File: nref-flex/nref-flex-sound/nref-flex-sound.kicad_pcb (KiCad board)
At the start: 2 copper layers, 6.5 x 115 mm, 3 parts, among them J1 Conn_01x10_Pin, J2 Conn_01x10_Pin

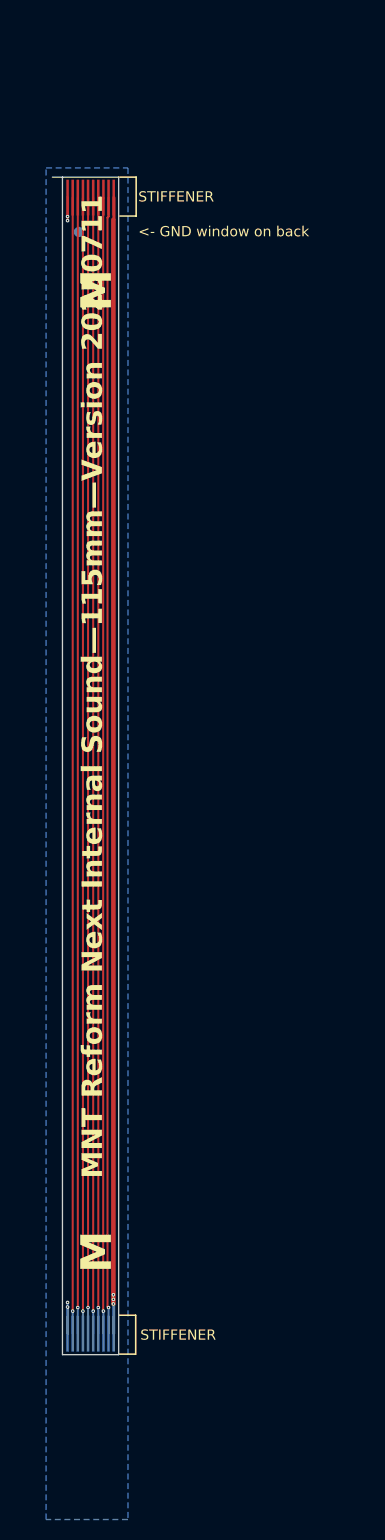
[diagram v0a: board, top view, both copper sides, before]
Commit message: commit various flex changes
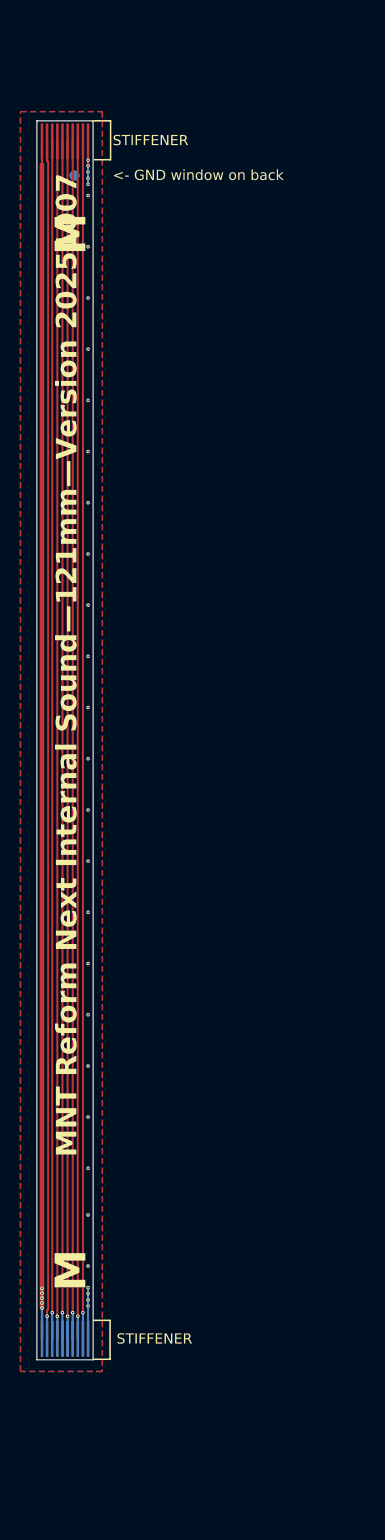
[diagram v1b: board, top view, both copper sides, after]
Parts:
- moved J1 6.04 mm to (85.7, 44.2), turned to 180 degrees
- moved TP1 5.53 mm to (86.6, 47.5)
- moved J2 2.55 mm to (85.7, 161.2), turned to 180 degrees
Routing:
- net +3V3: track 111.9 -> 118.7 mm, vias 3 -> 5
- net Net-(J1-Pin_8): track 111.0 -> 117.0 mm
- net Net-(J1-Pin_2): track 111.0 -> 117.0 mm
- net Net-(J1-Pin_9): track 111.0 -> 117.0 mm
- net Net-(J1-Pin_7): track 111.0 -> 117.0 mm
- net Net-(J1-Pin_6): track 111.0 -> 117.0 mm
- net Net-(J1-Pin_5): track 111.0 -> 117.0 mm
- net Net-(J1-Pin_4): track 111.0 -> 117.0 mm
- net Net-(J1-Pin_3): track 111.0 -> 117.0 mm
- net GND: track 8.10 -> 7.75 mm, vias 4 -> 31
- added copper zone on F.Cu, net GND
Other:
- board size 6.5 x 115 mm -> 5.5 x 121 mm
- board text added: "MNT Reform Next Internal Sound—121mm—Version 20251007"
- board text added: "target length: 121mm"
- board text removed: "MNT Reform Next Internal Sound—115mm—Version 20250711"
- board text removed: "trace w: 0.13, spacing: 0.2 target length: 115mm"
